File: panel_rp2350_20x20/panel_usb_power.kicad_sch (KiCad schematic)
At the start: 4 parts, among them J1 Conn_01x04, U43 AP2112K-3.3

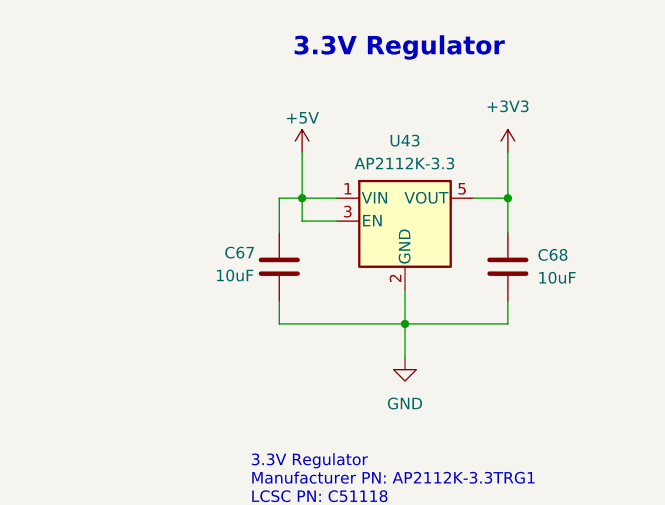
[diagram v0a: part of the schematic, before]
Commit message: Worked on setup for fabrication.
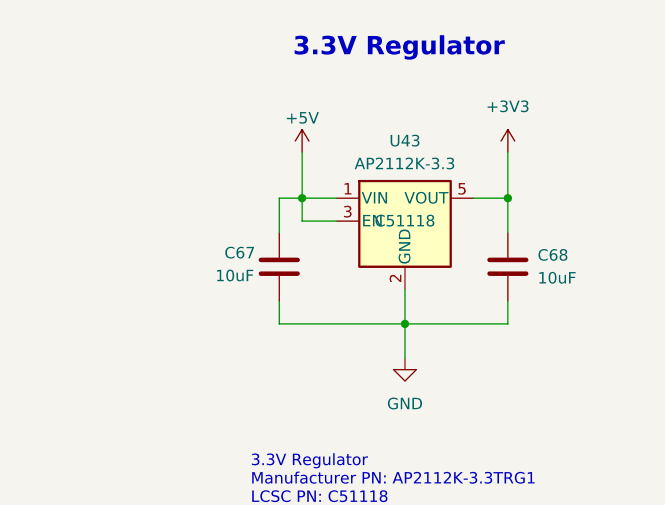
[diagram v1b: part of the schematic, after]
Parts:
- U43: LCSC Part # (none) -> C51118
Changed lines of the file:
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@@
+			)
+		)
+		(property "LCSC Part #" "C51118"
+			(at 214.63 48.26 0)
+			(effects
+				(font
+					(size 1.27 1.27)
+				)
 			)
 		)

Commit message: Worked on fab files.
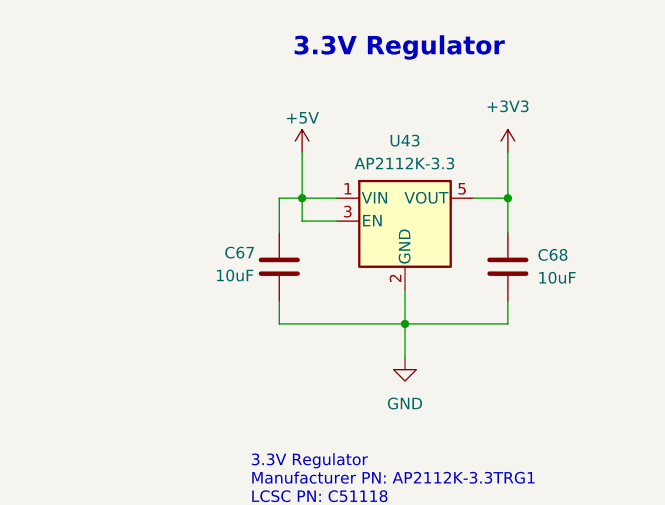
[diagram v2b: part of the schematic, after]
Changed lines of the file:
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@@
 					(size 1.27 1.27)
 				)
+				(hide yes)
 			)
 		)
